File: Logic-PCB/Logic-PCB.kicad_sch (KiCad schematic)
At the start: 55 parts, among them IC1 MC14027BDR2G, IC10 74LVC1G08FW5-7, IC11 MC14027BDR2G, IC12 TMUX4051PWR, IC13 TMUX4051PWR, IC14 TMUX4051PWR, IC15 TMUX4051PWR, IC16 TMUX4051PWR, IC17 TMUX4051PWR, IC18 TMUX4051PWR, IC19 TMUX4051PWR, IC2 LM555CMX_NOPB, IC3 NLV17SZ74USG, IC4 MC14043BDR2G, IC5 MC14027BDR2G, IC6 MC14027BDR2G, IC7 CD4082BM96, IC8 74LVC1G32GV,125, IC9 TMUX4051PWR, Q1 MMBT2222, SW1 SW_Push, SW2 SW_Push, SW3 SW_Push, SW4 SW_Push, SW5 SW_Push, SW6 SW_Push, SW7 SW_Push, SW8 SW_Push

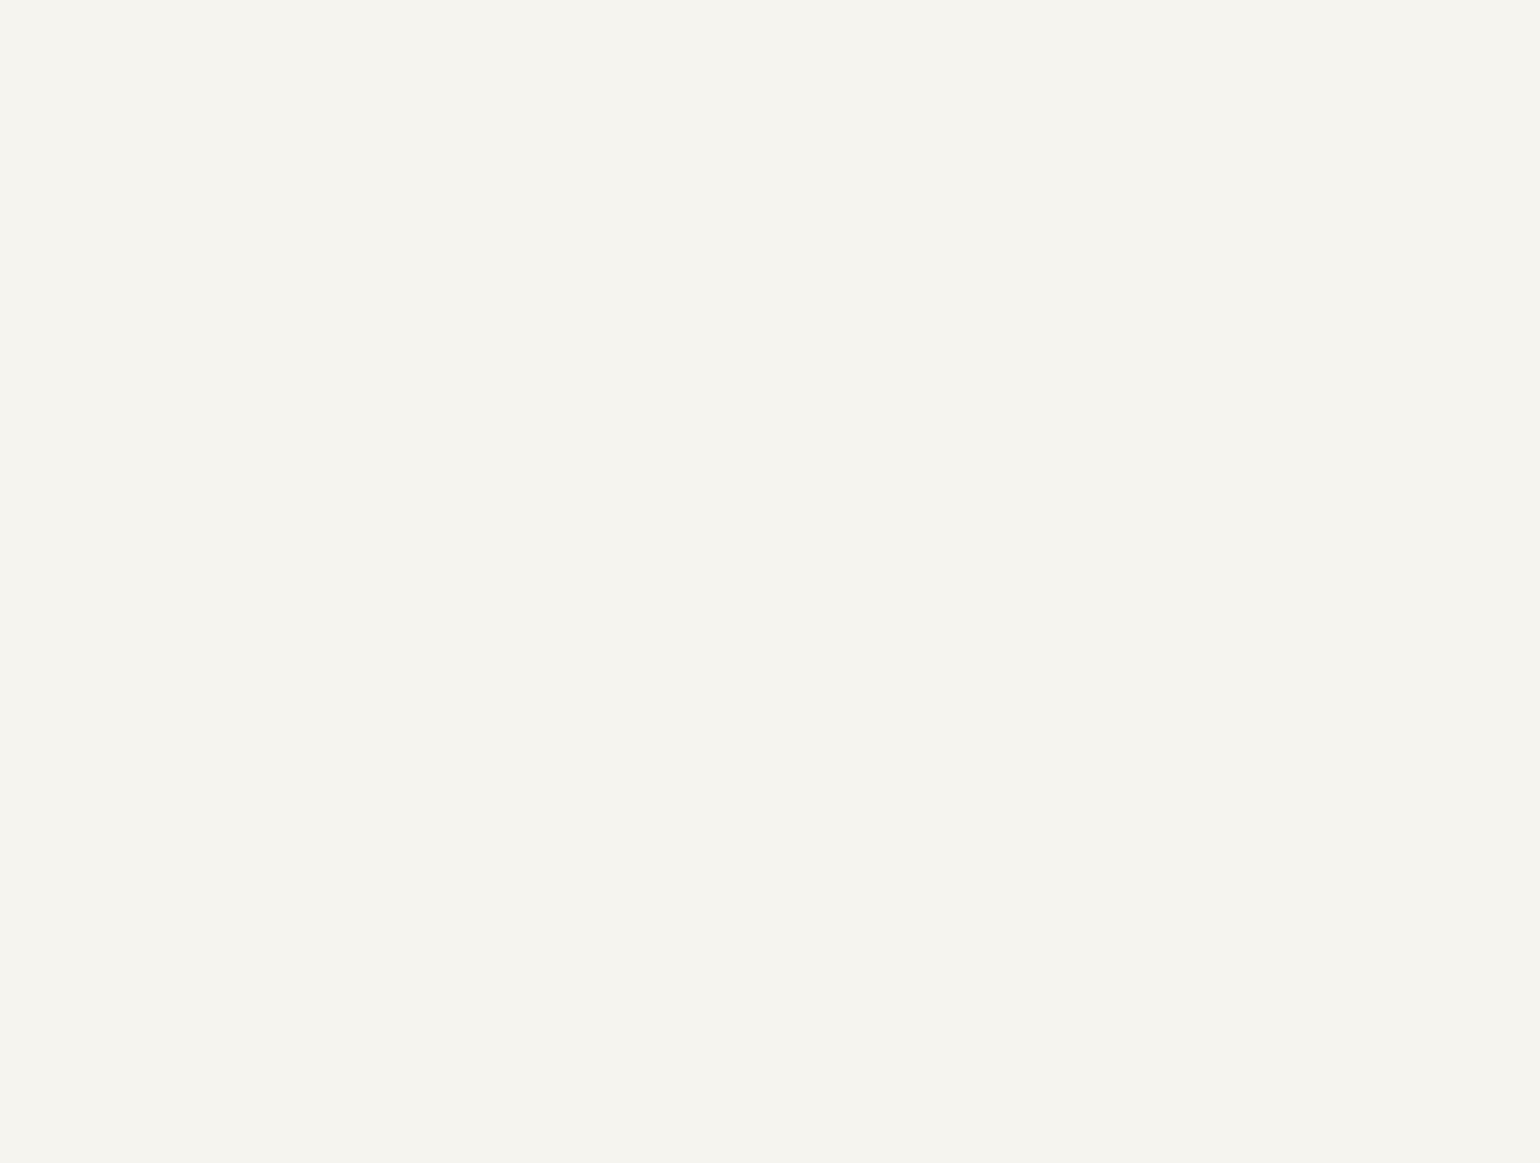
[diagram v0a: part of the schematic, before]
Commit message: gates
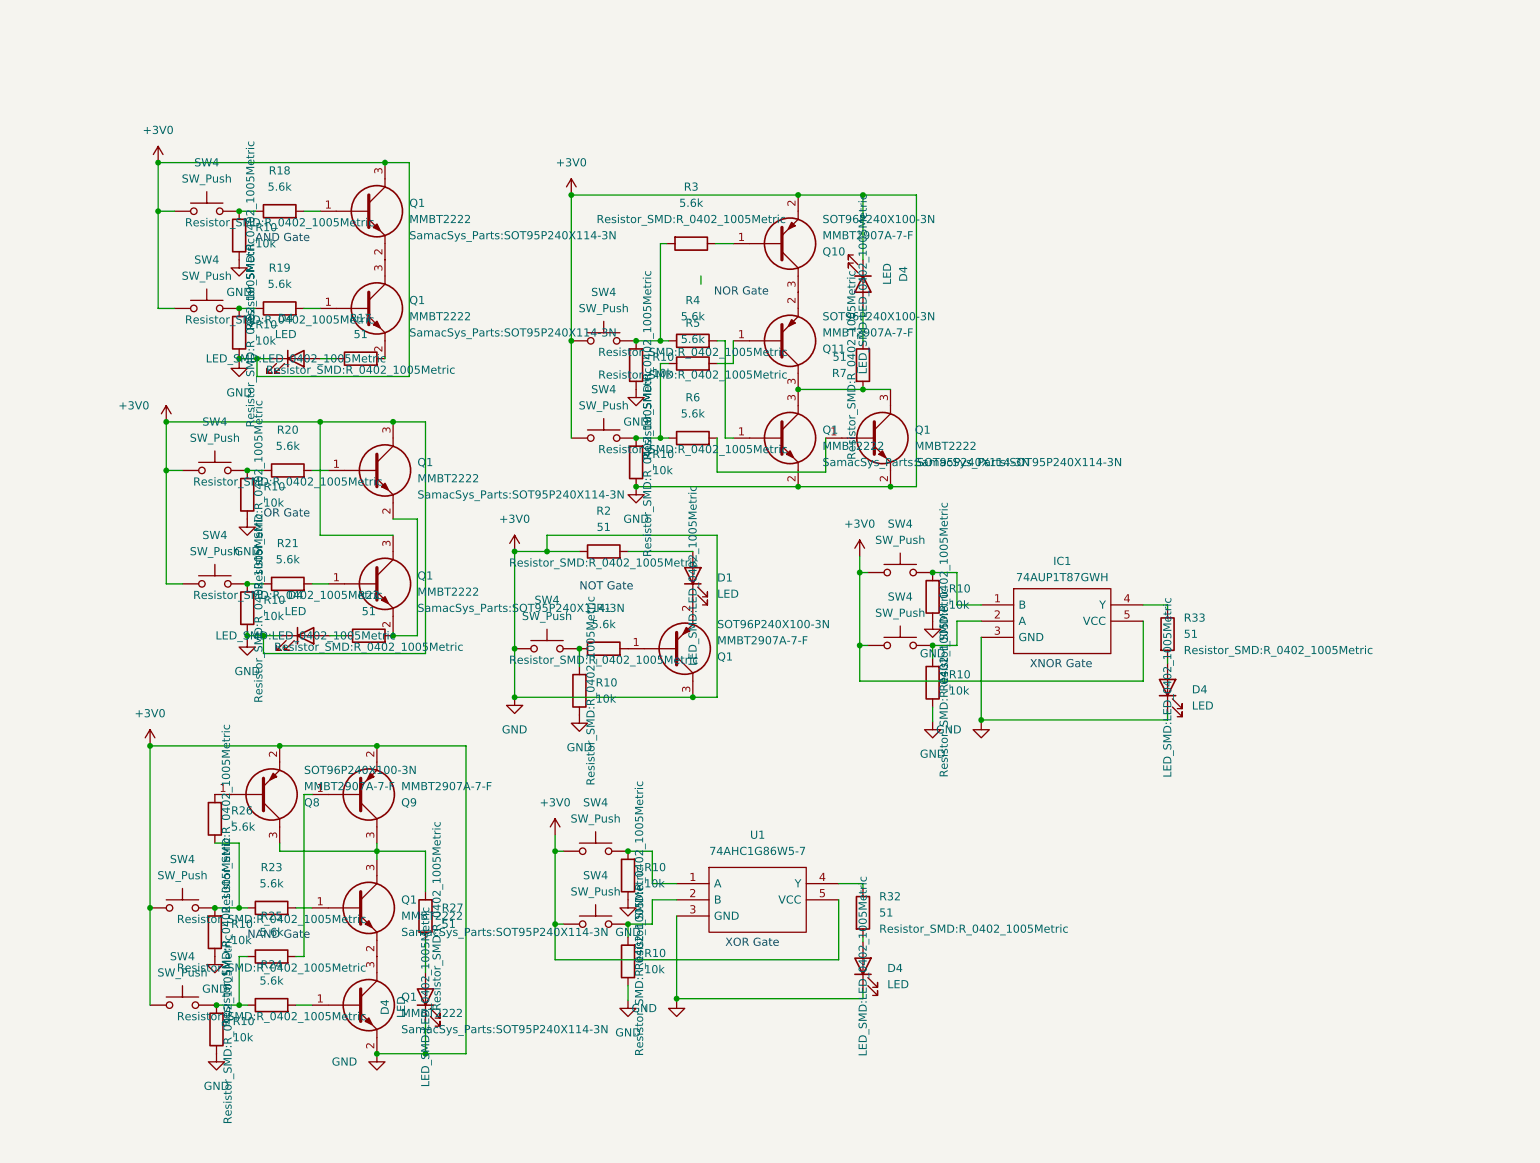
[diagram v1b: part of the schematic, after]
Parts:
- added D1, D4 (x6): LED, LED_SMD:LED_0402_1005Metric, symbol Device:LED
- added IC1: 74AUP1T87GWH, SOT65P212X110-5N, symbol SamacSys_Parts:74AUP1T87GWH
- added Q1 (x8): MMBT2222, SamacSys_Parts:SOT95P240X114-3N, symbol SamacSys_Parts:MMBT2222
- added Q1, Q10, Q11, Q8, Q9: MMBT2907A-7-F, SOT96P240X100-3N, symbol SamacSys_Parts:MMBT2907A-7-F
- added R1, R18, R19, R20, R21, R23, R24, R25, R26, R3, R4, R5, R6: 5.6k, Resistor_SMD:R_0402_1005Metric, symbol Device:R
- added R10 (x13): 10k, Resistor_SMD:R_0402_1005Metric, symbol Device:R
- added R17, R2, R22, R27, R32, R33, R7: 51, Resistor_SMD:R_0402_1005Metric, symbol Device:R
- added SW4 (x13): SW_Push, symbol Switch:SW_Push
- added U1: 74AHC1G86W5-7, SOT95P285X130-5N, symbol SamacSys_Parts:74AHC1G86W5-7
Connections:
- net GND is gone; now on net +3V0: C1.2, C2.2, C3.2, D1.1 (K), D2.1 (K), D3.1 (K), D4.1 (K), D5.1 (K), D6.1 (K), IC1.4 (RA), IC1.7 (SA), IC1.8 (VSS), IC10.3 (GND), IC11.4 (RA), IC11.7 (SA), IC11.8 (VSS), IC12.1 (S4), IC12.12 (S3), IC12.13 (S0), IC12.14 (S1), IC12.2 (S6), IC12.4 (S7), IC12.5 (S5), IC12.6 (~{EN}), IC12.7 (VSS), IC12.8 (GND), IC13.1 (S4), IC13.12 (S3), IC13.14 (S1), IC13.2 (S6), IC13.4 (S7), IC13.5 (S5), IC13.6 (~{EN}), IC13.7 (VSS), IC13.8 (GND), IC14.6 (~{EN}), IC14.7 (VSS), IC14.8 (GND), IC15.6 (~{EN}), IC15.7 (VSS), IC15.8 (GND), IC16.6 (~{EN}), IC16.7 (VSS), IC16.8 (GND), IC17.6 (~{EN}), IC17.7 (VSS), IC17.8 (GND), IC18.6 (~{EN}), IC18.7 (VSS), IC18.8 (GND), IC19.6 (~{EN}), IC19.7 (VSS), IC19.8 (GND), IC2.1 (GND), IC3.4 (GND), IC4.8 (VSS), IC5.4 (RA), IC5.7 (SA), IC5.8 (VSS), IC6.12 (RB), IC6.4 (RA), IC6.7 (SA), IC6.8 (VSS), IC6.9 (SB), IC7.7 (VSS), IC8.3 (GND), IC9.15 (S2), IC9.2 (S6), IC9.4 (S7), IC9.5 (S5), IC9.6 (~{EN}), IC9.7 (VSS), IC9.8 (GND), Q1.2, R10.1, R12.1, R13.1, R14.1, R16.1, R8.1, R9.1
- net +3V0: now also D4.1 (K), D4.1 (K), D4.1 (K), D4.1 (K), D4.1 (K), D4.1 (K), IC1.3 (GND), IC1.5 (VCC), Q1.2, Q1.2, Q1.2, Q1.3, Q1.3, Q1.3, Q1.3, Q10.2, Q8.2, Q9.2, R10.1, R10.1, R10.1, R10.1, R10.1, R10.1, R10.1, R10.1, R10.1, R10.1, R10.1, R10.1, R10.1, R2.1, SW4.1, SW4.1, SW4.1, SW4.1, SW4.1, SW4.1, SW4.1, SW4.1, SW4.1, SW4.1, SW4.1, SW4.1, SW4.1, U1.3 (GND), U1.5 (VCC)
- new net: R1.1, R10.2, SW4.2
- new net: R10.2, R5.1, R6.1, SW4.2
- new net: Q1.1, R6.2
- new net: D4.2 (A), R27.1
- new net: D4.2 (A), R32.2
- new net: R10.2, SW4.2, U1.1 (A)
- new net: Q10.1, R3.1
- new net: R10.2, R3.2, R4.1, SW4.2
- new net: D1.1 (K), Q1.2
- new net: D1.2 (A), R2.2
- new net: R10.2, R19.1, SW4.2
- new net: R10.2, R18.1, SW4.2
- new net: Q1.1, R18.2
- new net: Q1.2, Q1.3 (x2)
- new net: R10.2, R23.1, R26.1, SW4.2
- new net: Q8.1, R26.2
- new net: IC1.4 (Y), R33.1
- new net: D4.2 (A), R33.2
- new net: R10.2, R21.1, SW4.2
- new net: IC1.2 (A), R10.2, SW4.2
- new net: IC1.1 (B), R10.2, SW4.2
- new net: Q1.1, R20.2
- new net: Q1.2, Q1.2, R22.2
- new net: R10.2, R20.1, SW4.2
- new net: D4.2 (A), R7.1
- new net: Q1.3, Q1.3, Q11.3, R7.2
- new net: Q1.1, R21.2
- new net: R10.2, R24.1, R25.1, SW4.2
- new net: Q9.1, R25.2
- new net: D4.2 (A), R22.1
- new net: Q10.3, Q11.2
- new net: Q11.1, R5.2
- new net: Q1.1, R23.2
- new net: Q1.1, R19.2
- new net: Q1.3, Q8.3, Q9.3, R27.2
- new net: Q1.1, R24.2
- new net: R10.2, SW4.2, U1.2 (B)
- new net: D4.2 (A), R17.1
- new net: Q1.2, R17.2
- new net: R32.1, U1.4 (Y)
- new net: Q1.1, R4.2
- new net: Q1.1, R1.2
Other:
- note added: "AND Gate"
- note added: "NAND Gate"
- note added: "NOR Gate"
- note added: "NOT Gate"
- note added: "OR Gate"
- note added: "XNOR Gate"
- note added: "XOR Gate"

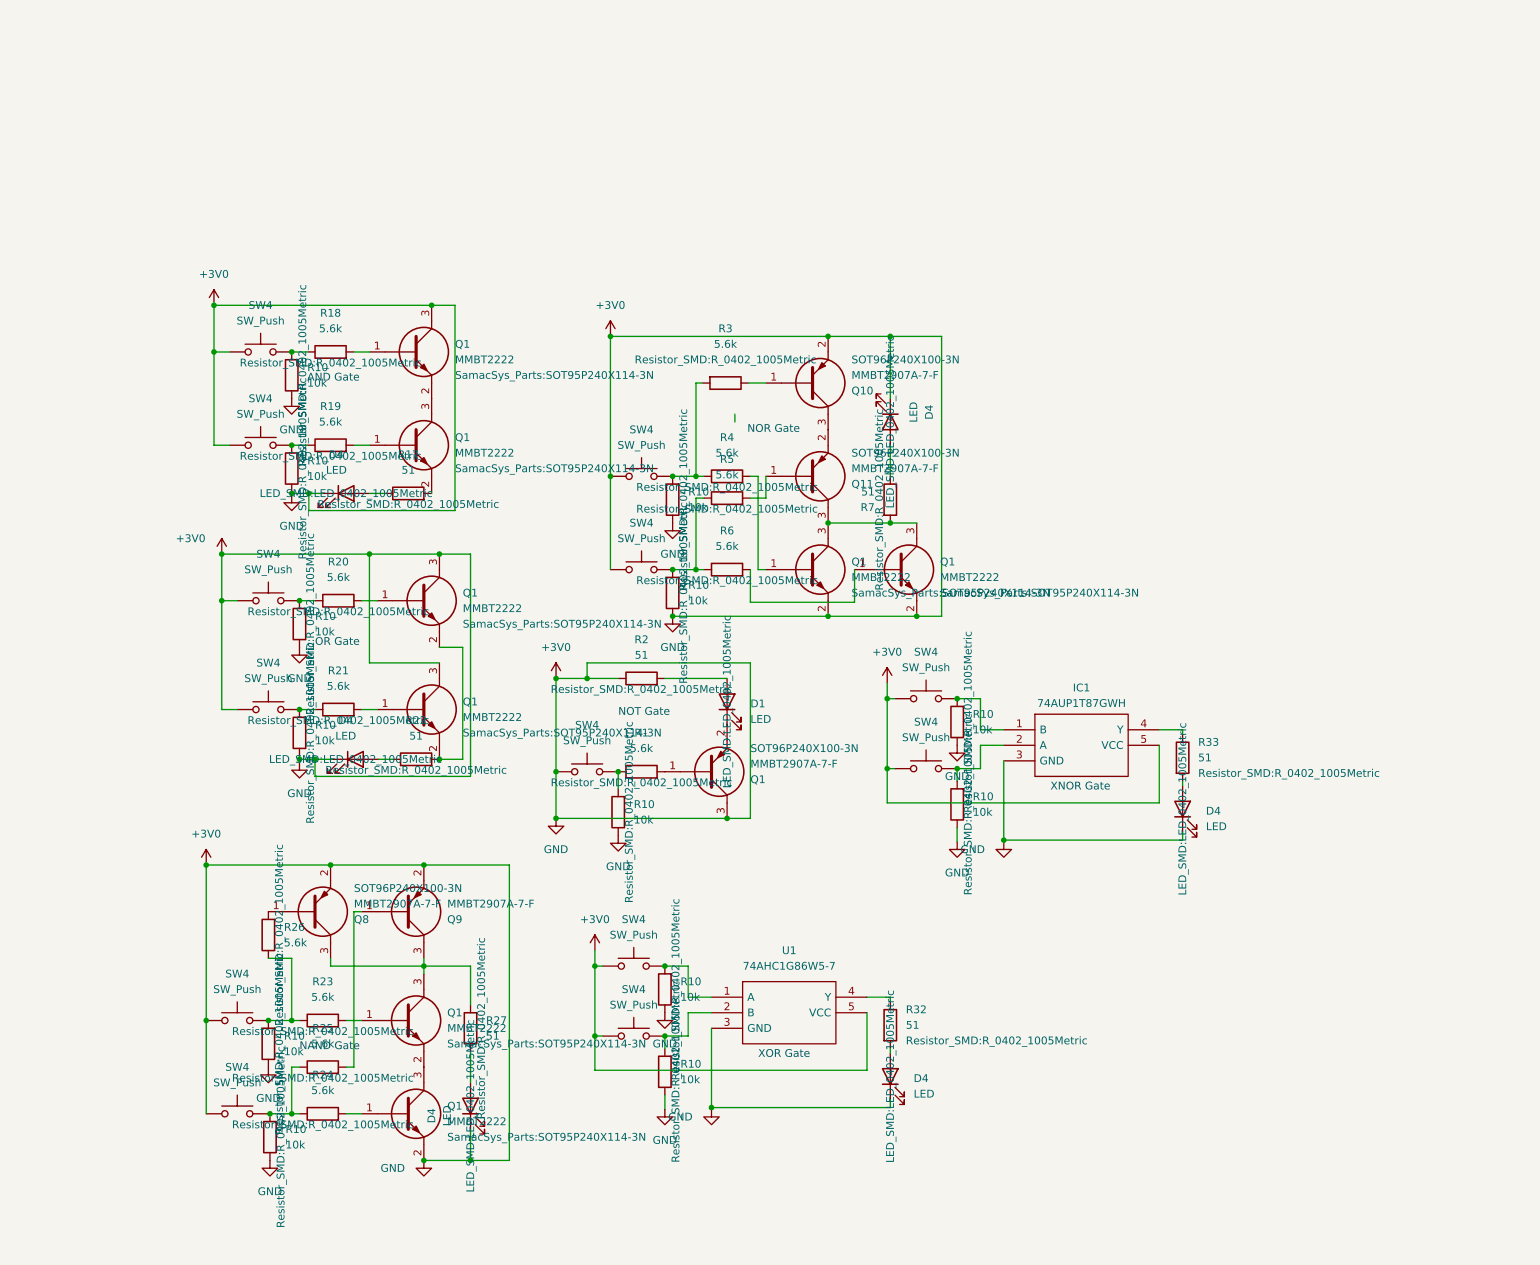
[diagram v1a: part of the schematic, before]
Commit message: Update Logic-PCB.kicad_sch
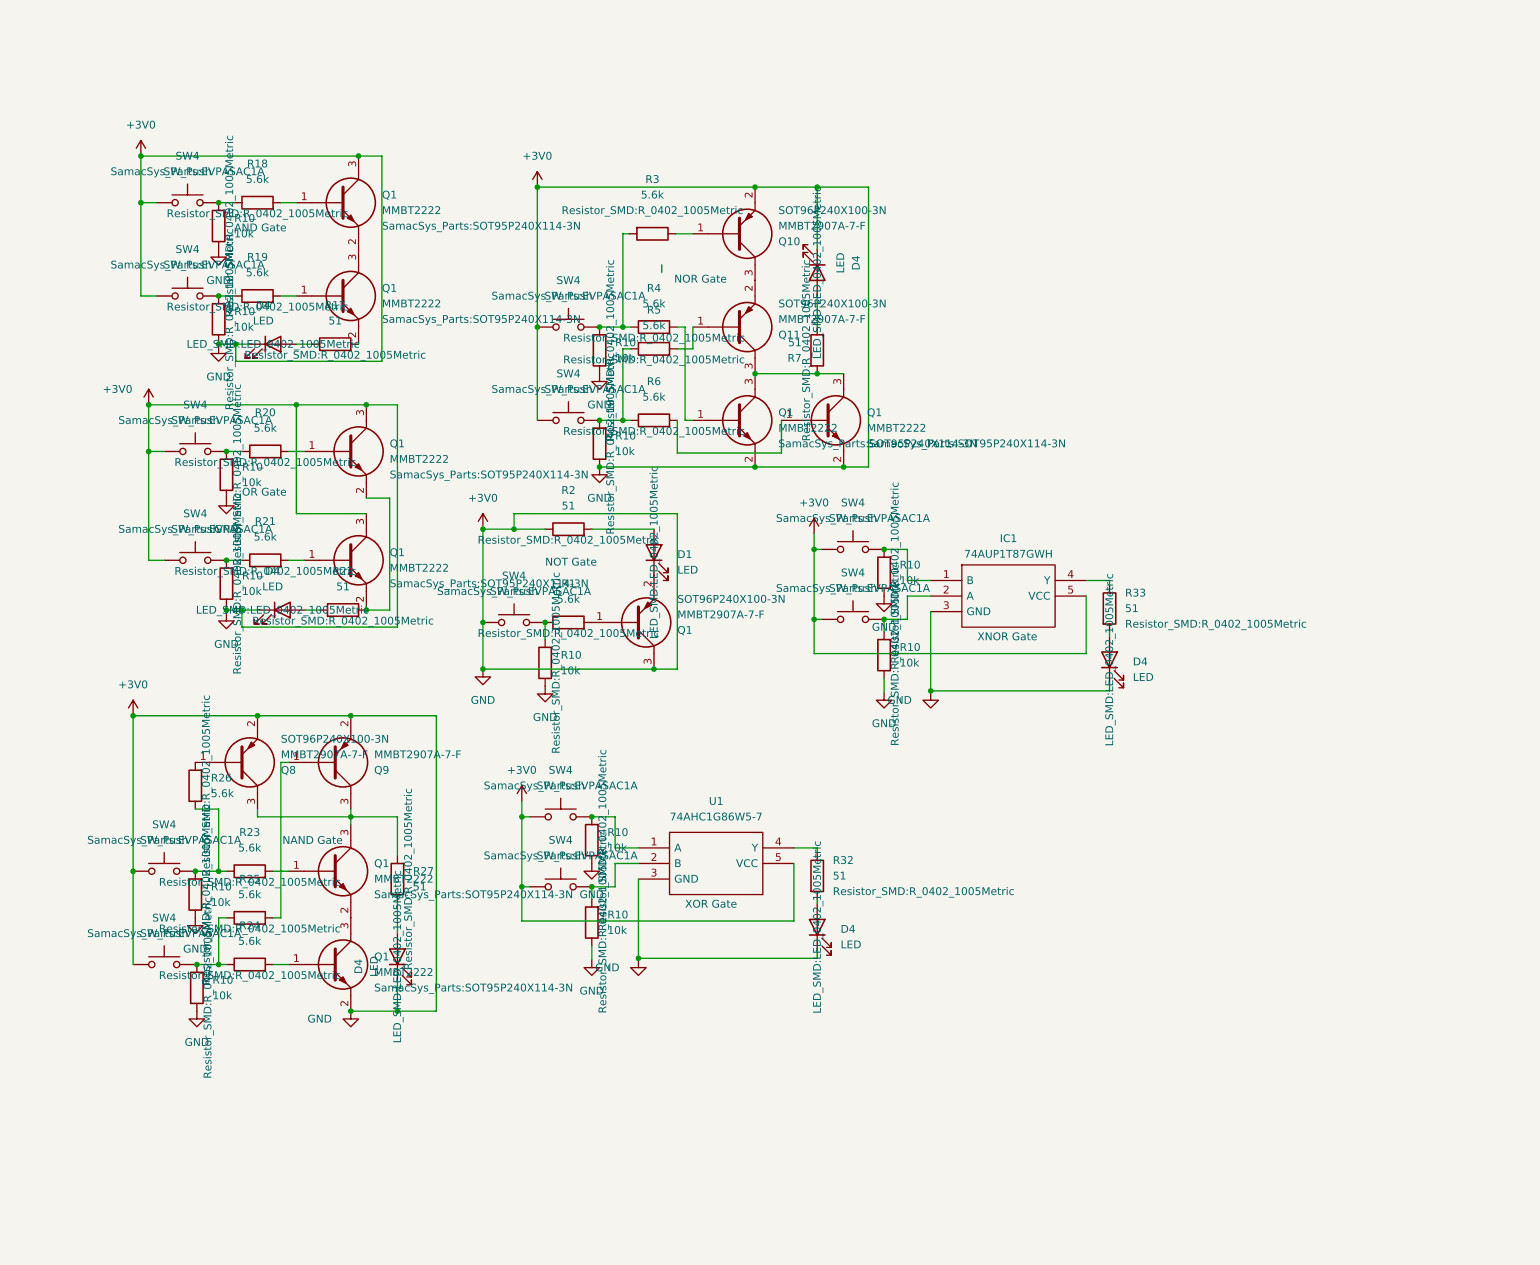
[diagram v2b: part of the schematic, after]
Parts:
- removed D4 (x6): LED, LED_SMD:LED_0402_1005Metric, symbol Device:LED
- removed Q1 (x8): MMBT2222, SamacSys_Parts:SOT95P240X114-3N, symbol SamacSys_Parts:MMBT2222
- removed R10 (x13): 10k, Resistor_SMD:R_0402_1005Metric, symbol Device:R
- removed SW4 (x13): SW_Push, symbol Switch:SW_Push
- added D4 (x6): LED, LED_SMD:LED_0402_1005Metric, symbol Device:LED
- added Q1 (x8): MMBT2222, SamacSys_Parts:SOT95P240X114-3N, symbol SamacSys_Parts:MMBT2222
- added R10 (x13): 10k, Resistor_SMD:R_0402_1005Metric, symbol Device:R
- added SW4 (x13): SW_Push, SamacSys_Parts:EVPASAC1A, symbol Switch:SW_Push
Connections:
- net +3V0: now also D4.1 (K), D4.1 (K), D4.1 (K), D4.1 (K), D4.1 (K), D4.1 (K), Q1.2, Q1.2, Q1.2, Q1.3, Q1.3, Q1.3, R10.1, R10.1, R10.1, R10.1, R10.1, R10.1, R10.1, R10.1, R10.1, R10.1, R10.1, R10.1, R10.1, SW4.1, SW4.1, SW4.1, SW4.1, SW4.1, SW4.1, SW4.1, SW4.1, SW4.1, SW4.1, SW4.1, SW4.1, SW4.1
- net at R1.1: now also R10.2, SW4.2
- net at R5.1, R6.1: now also R10.2, SW4.2
- net at R6.2: now also Q1.1
- net at R27.1: now also D4.2 (A)
- net at R32.2: now also D4.2 (A)
- net at U1.1 (A): now also R10.2, SW4.2
- net at R3.2, R4.1: now also R10.2, SW4.2
- net at R19.1: now also R10.2, SW4.2
- net at R18.1: now also R10.2, SW4.2
- net at R18.2: now also Q1.1
- net at R23.1, R26.1: now also R10.2, SW4.2
- net at R33.2: now also D4.2 (A)
- net at R21.1: now also R10.2, SW4.2
- net at IC1.2 (A): now also R10.2, SW4.2
- net at IC1.1 (B): now also R10.2, SW4.2
- net at R20.2: now also Q1.1
- net at R22.2: now also Q1.2, Q1.2
- net at R20.1: now also R10.2, SW4.2
- net at R7.1: now also D4.2 (A)
- net at Q11.3, R7.2: now also Q1.3, Q1.3
- net at R21.2: now also Q1.1
- net at R24.1, R25.1: now also R10.2, SW4.2
- net at R22.1: now also D4.2 (A)
- net at R23.2: now also Q1.1
- net at R19.2: now also Q1.1
- net at Q8.3, Q9.3, R27.2: now also Q1.3
- net at R24.2: now also Q1.1
- net at U1.2 (B): now also R10.2, SW4.2
- net at R17.1: now also D4.2 (A)
- net at R17.2: now also Q1.2
- net at R4.2: now also Q1.1
- new net: Q1.2, Q1.3 (x2)
